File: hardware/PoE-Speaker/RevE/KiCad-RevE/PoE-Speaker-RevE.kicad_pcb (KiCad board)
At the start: 4 copper layers, 210 x 100 mm, 209 parts, among them J1 2250506-1, J2 MX2EDGR-5.08-02P-GN01-Cu-A, J3 MX2EDGR-5.08-02P-GN01-Cu-A, J4 Pin Header 02x07 2.54mm Verti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, J5 Pin Header 01x06 2.54mm Verti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, J6 Pin Header 01x06 2.54mm Verti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, Q1 DMNH6012LK3-13, Q2 DMNH6012LK3-13, Q3 PSMN4R8-100BSE, Q4 PSMN4R8-100BSE, SW1 TS-1088-AR02016, SW2 TS-1088-AR02016, U1 Ag5800, U10 LM5050-2, U11 PCAL6416APW, U12 PC817X2NSZ9F, U13 PC817X2NSZ9F, U14 PC817X2NSZ9F, U15 LTC4365HTS8#TRPBF, U16 TPS26630RGER, U2 ESP32-S3-WROOM-1U-N16R8, U3 W5500, U4 PCM5122PWR, U5 TPA3116D2, U6 LMR33630AQRNXRQ1, U7 TPS62132RGTR, U8 RT9013-33GB, U9 LM5050-2, X2 25MHz

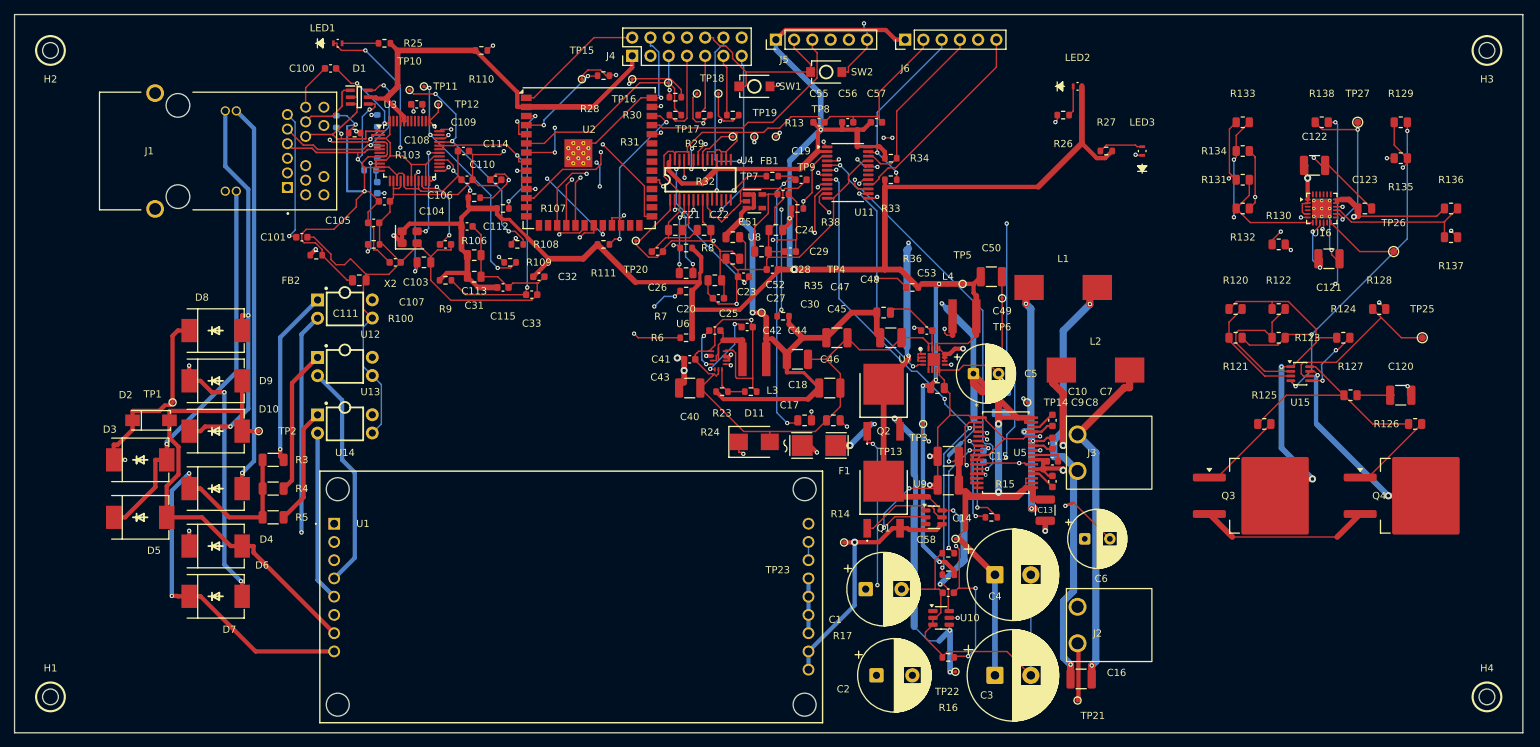
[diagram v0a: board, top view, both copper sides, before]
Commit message: docs: archive final engineered PCB handoffs
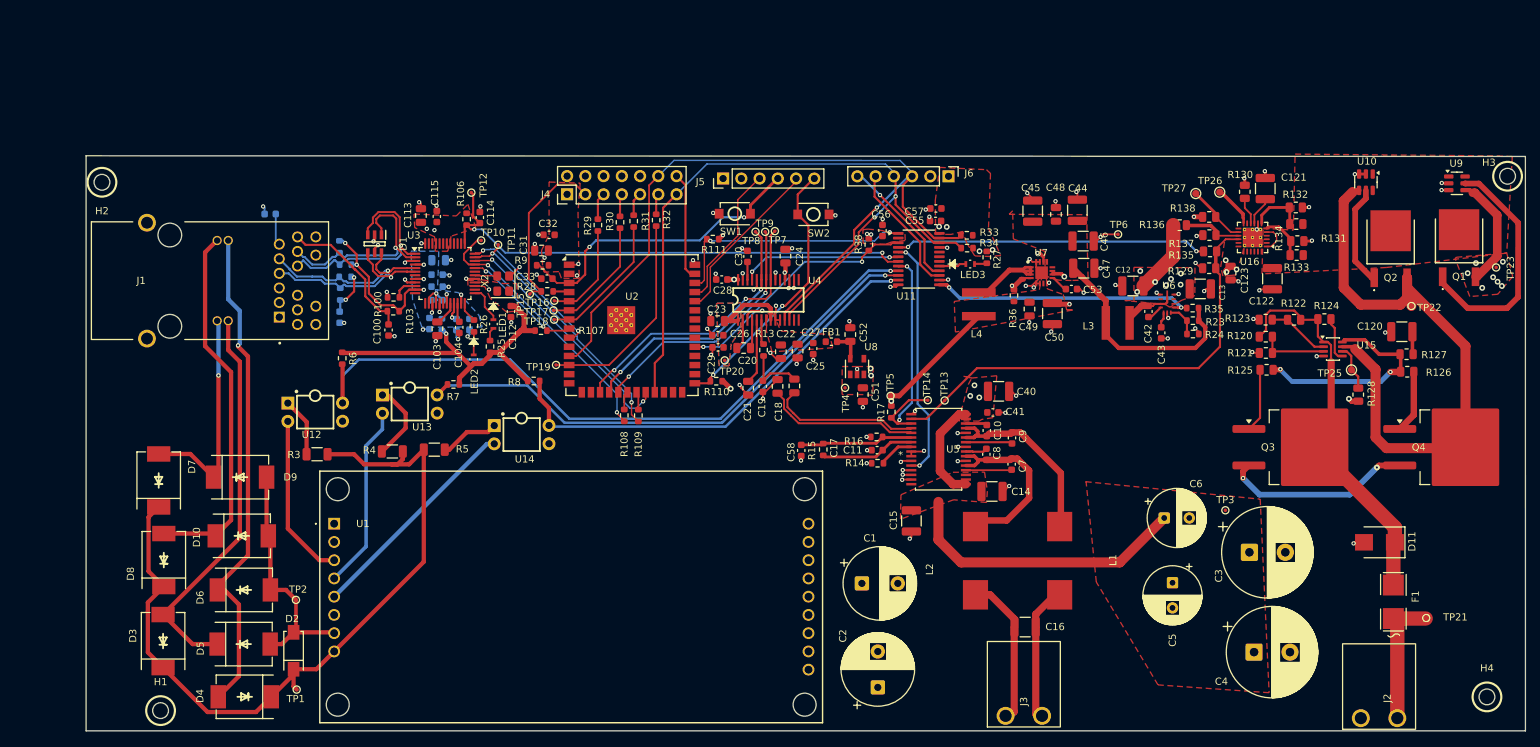
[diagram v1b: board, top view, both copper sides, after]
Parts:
- C101, C105, C106, C107, C108, C109, C110, C111, FB2: moved to B.Cu
- C11, C12: moved to F.Cu
- moved TP23 98.5 mm to (276.3, 85.2)
- moved LED2 92.3 mm to (133.9, 98.0), turned to -90 degrees
- moved D11 88.1 mm to (260.0, 123.5), turned to 180 degrees
- moved Q1 87.4 mm to (271.1, 82.5)
- moved R26 87.1 mm to (134.0, 93.4), turned to -90 degrees
- moved U9 86.4 mm to (270.8, 73.5)
- moved U10 84.7 mm to (258.1, 73.3), turned to -90 degrees
- moved F1 82.9 mm to (262.0, 131.8), turned to 90 degrees
- moved TP22 81.4 mm to (264.5, 90.6)
- moved Q2 73.8 mm to (261.6, 82.6)
- moved R23 66.3 mm to (234.1, 92.6), turned to 180 degrees
- moved U6 63.0 mm to (230.5, 90.1)
- moved R24 62.1 mm to (234.1, 94.5)
- moved C42 60.4 mm to (227.9, 91.3), turned to 90 degrees
- moved C43 57.7 mm to (229.7, 94.3), turned to -90 degrees
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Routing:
- net GND: track 956.0 -> 133.3 mm, vias 28 -> 110
- net 3V3: track 549.7 -> 290.7 mm, vias 14 -> 22
- net 24V_AMP: track 281.8 -> 112.0 mm, vias 9 -> 13
- net 24V_OR: track 140.2 -> 4.04 mm, vias 6 -> 0
- net 24V_POE: track 45.1 -> 148.6 mm, vias 1 -> 7
- net PHY_SPEED_LED: track 95.3 -> 2.85 mm, vias 6 -> 0
- net BENCH_FUSED: track 140.0 -> 55.5 mm, vias 5 -> 0
- net ETH_3V3A: track 97.4 -> 28.0 mm, vias 4 -> 8
- net BOOT_GPIO0: track 102.6 -> 38.0 mm, vias 3 -> 2
- net AMP_SDZ: track 123.3 -> 64.7 mm, vias 6 -> 0
- net 24V_BENCH_PROTECTED: track 138.8 -> 84.7 mm, vias 5 -> 0
- net 5V: track 118.8 -> 66.0 mm
- net 3V3A: track 59.2 -> 10.5 mm, vias 2 -> 0
- net AMP_FAULTZ: track 79.1 -> 33.4 mm, vias 5 -> 2
- net ESP_EN: track 84.8 -> 43.2 mm, vias 3 -> 2
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- added copper zone on F.Cu, net 24V_AMP
- added copper zone on In2.Cu, net 24V_AMP
- added copper zone on F.Cu, net 24V_OR
- added copper zone on F.Cu, net 24V_POE
- added copper zone on In2.Cu, net 24V_POE
- added copper zone on F.Cu, net 3V3
- added copper zone on B.Cu, net 3V3A
- added copper zone on F.Cu, net 3V3A
- added copper zone on F.Cu, net 5V
- added copper zone on B.Cu, net ETH_3V3A
- added copper zone on In2.Cu, net POE_12V_MID
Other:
- board size 210 x 100 mm -> 200.4 x 80.1 mm
